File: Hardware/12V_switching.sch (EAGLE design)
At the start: 9 parts, among them IC5 LM2576HVSX-12/NOPB, J1 POWERPOLE_POWER45A, J2 POWERPOLE_POWER45A, J3 POWERPOLE_POWER45A

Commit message: Fix a non connected network on the board... the motor VOut .. :(
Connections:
- net +VIN: now also J3.V+
- net GND: now also J3.GND
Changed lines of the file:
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@@
 <wire x1="160.02" y1="0" x2="162.56" y2="0" width="0.1524" layer="91"/>
 <label x="160.02" y="0" size="1.016" layer="95" rot="MR0" xref="yes"/>
+<pinref part="J3" gate="G$1" pin="GND"/>
 </segment>
 </net>
@@
 <wire x1="160.02" y1="10.16" x2="162.56" y2="10.16" width="0.1524" layer="91"/>
 <label x="160.02" y="10.16" size="1.016" layer="95" rot="MR0" xref="yes"/>
+<pinref part="J3" gate="G$1" pin="V+"/>
 </segment>
 </net>

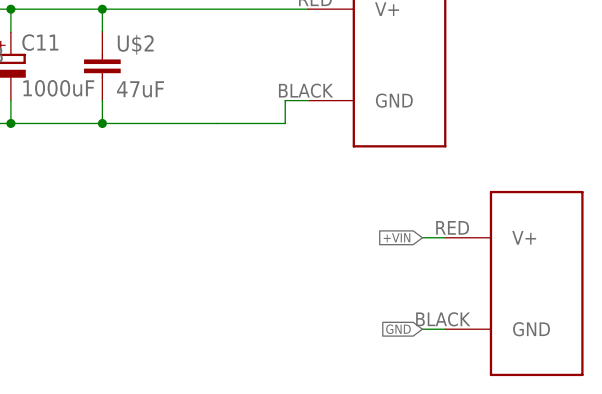
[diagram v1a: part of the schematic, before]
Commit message: Update some of the components on the 12V adapter.
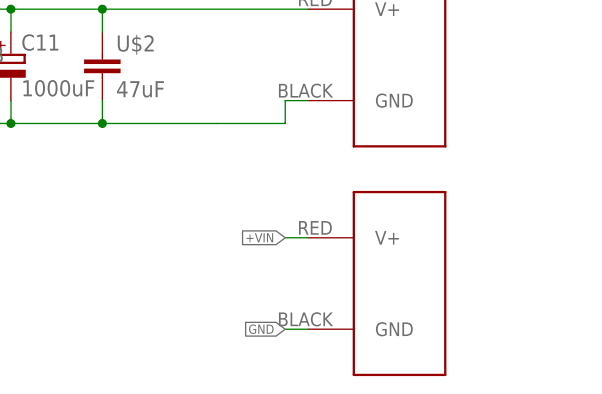
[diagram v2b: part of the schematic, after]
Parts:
- C10, C11: device rcl:CPOL-EUUD-10X10 -> rti:CPOL-EU
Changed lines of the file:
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@@
 <part name="D2" library="diode" deviceset="DIODE-" device="DO-214AC" value="SAC34"/>
 <part name="L1" library="MSS1583-104KEB" deviceset="MSS1583-104KEB" device=""/>
-<part name="C10" library="rcl" deviceset="CPOL-EU" device="UD-10X10" value="100uF 100V"/>
-<part name="C11" library="rcl" deviceset="CPOL-EU" device="UD-10X10" value="1000uF"/>
+<part name="C10" library="rti" deviceset="CPOL-EU" device="" value="100uF 100V"/>
+<part name="C11" library="rti" deviceset="CPOL-EU" device="" value="1000uF"/>
 <part name="U$2" library="rti" deviceset="C-EU" device="'1206'" value="47uF"/>
 <part name="J1" library="powerpoles" deviceset="POWERPOLE_POWER" device="45A"/>
@@
 <instance part="J1" gate="G$1" x="10.16" y="48.26" rot="R180"/>
 <instance part="J2" gate="G$1" x="157.48" y="30.48"/>
-<instance part="J3" gate="G$1" x="172.72" y="5.08"/>
+<instance part="J3" gate="G$1" x="157.48" y="5.08"/>
 </instances>
 <busses>
@@
 </segment>
 <segment>
-<wire x1="160.02" y1="0" x2="162.56" y2="0" width="0.1524" layer="91"/>
-<label x="160.02" y="0" size="1.016" layer="95" rot="MR0" xref="yes"/>
+<wire x1="144.78" y1="0" x2="147.32" y2="0" width="0.1524" layer="91"/>
+<label x="144.78" y="0" size="1.016" layer="95" rot="MR0" xref="yes"/>
 <pinref part="J3" gate="G$1" pin="GND"/>
 </segment>
@@
 </segment>
 <segment>
-<wire x1="160.02" y1="10.16" x2="162.56" y2="10.16" width="0.1524" layer="91"/>
-<label x="160.02" y="10.16" size="1.016" layer="95" rot="MR0" xref="yes"/>
+<wire x1="144.78" y1="10.16" x2="147.32" y2="10.16" width="0.1524" layer="91"/>
+<label x="144.78" y="10.16" size="1.016" layer="95" rot="MR0" xref="yes"/>
 <pinref part="J3" gate="G$1" pin="V+"/>
 </segment>

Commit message: Fix merge conflict
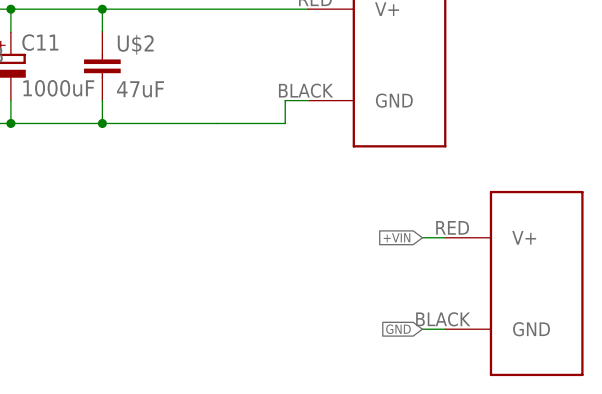
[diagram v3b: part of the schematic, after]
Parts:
- C10, C11: device rti:CPOL-EU -> rcl:CPOL-EUUD-10X10
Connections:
- net +VIN: no longer J3.V+
- net GND: no longer J3.GND
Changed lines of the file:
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@@
 <part name="D2" library="diode" deviceset="DIODE-" device="DO-214AC" value="SAC34"/>
 <part name="L1" library="MSS1583-104KEB" deviceset="MSS1583-104KEB" device=""/>
-<part name="C10" library="rti" deviceset="CPOL-EU" device="" value="100uF 100V"/>
-<part name="C11" library="rti" deviceset="CPOL-EU" device="" value="1000uF"/>
+<part name="C10" library="rcl" deviceset="CPOL-EU" device="UD-10X10" value="100uF 100V"/>
+<part name="C11" library="rcl" deviceset="CPOL-EU" device="UD-10X10" value="1000uF"/>
 <part name="U$2" library="rti" deviceset="C-EU" device="'1206'" value="47uF"/>
 <part name="J1" library="powerpoles" deviceset="POWERPOLE_POWER" device="45A"/>
@@
 <instance part="J1" gate="G$1" x="10.16" y="48.26" rot="R180"/>
 <instance part="J2" gate="G$1" x="157.48" y="30.48"/>
-<instance part="J3" gate="G$1" x="157.48" y="5.08"/>
+<instance part="J3" gate="G$1" x="172.72" y="5.08"/>
 </instances>
 <busses>
@@
 </segment>
 <segment>
-<wire x1="144.78" y1="0" x2="147.32" y2="0" width="0.1524" layer="91"/>
-<label x="144.78" y="0" size="1.016" layer="95" rot="MR0" xref="yes"/>
-<pinref part="J3" gate="G$1" pin="GND"/>
+<wire x1="160.02" y1="0" x2="162.56" y2="0" width="0.1524" layer="91"/>
+<label x="160.02" y="0" size="1.016" layer="95" rot="MR0" xref="yes"/>
 </segment>
 </net>
@@
 </segment>
 <segment>
-<wire x1="144.78" y1="10.16" x2="147.32" y2="10.16" width="0.1524" layer="91"/>
-<label x="144.78" y="10.16" size="1.016" layer="95" rot="MR0" xref="yes"/>
-<pinref part="J3" gate="G$1" pin="V+"/>
+<wire x1="160.02" y1="10.16" x2="162.56" y2="10.16" width="0.1524" layer="91"/>
+<label x="160.02" y="10.16" size="1.016" layer="95" rot="MR0" xref="yes"/>
 </segment>
 </net>
